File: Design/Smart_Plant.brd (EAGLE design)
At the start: 80 x 129.1 mm, 69 parts, among them IC1 TP4056, IC2 TLC555CDR, IC3 AHT20, IC4 RT9080-33GJ5, J6 USB-C, Q1 IRLML0100, T1 MMBT2222A, T2 LBSS84LT1G, U2 ESP32-WROOM-32

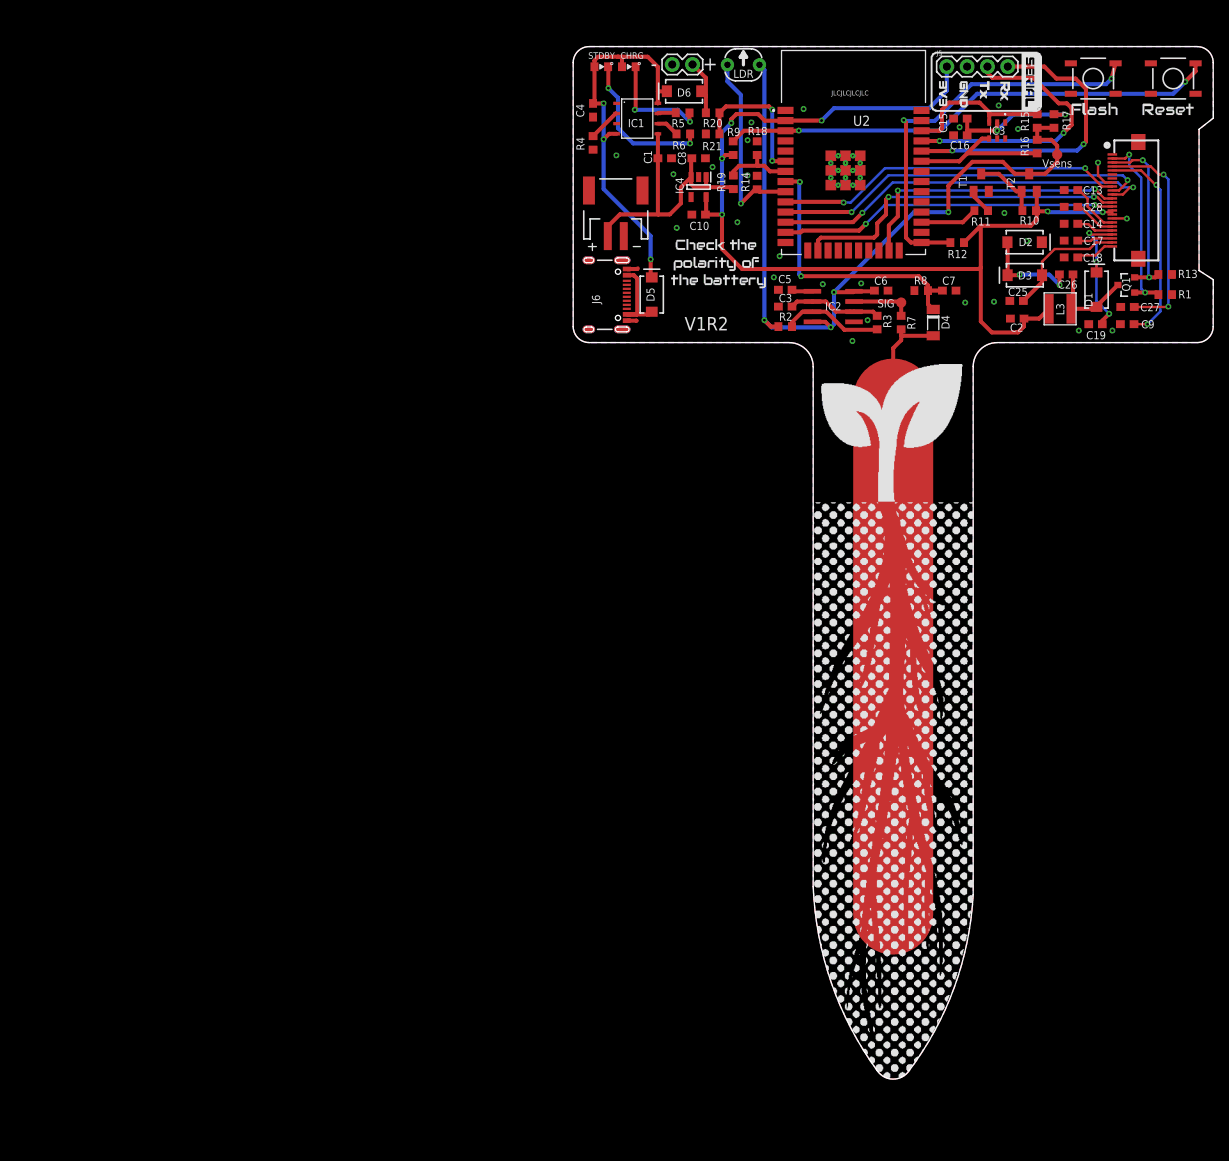
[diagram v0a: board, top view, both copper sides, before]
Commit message: SoC first draft
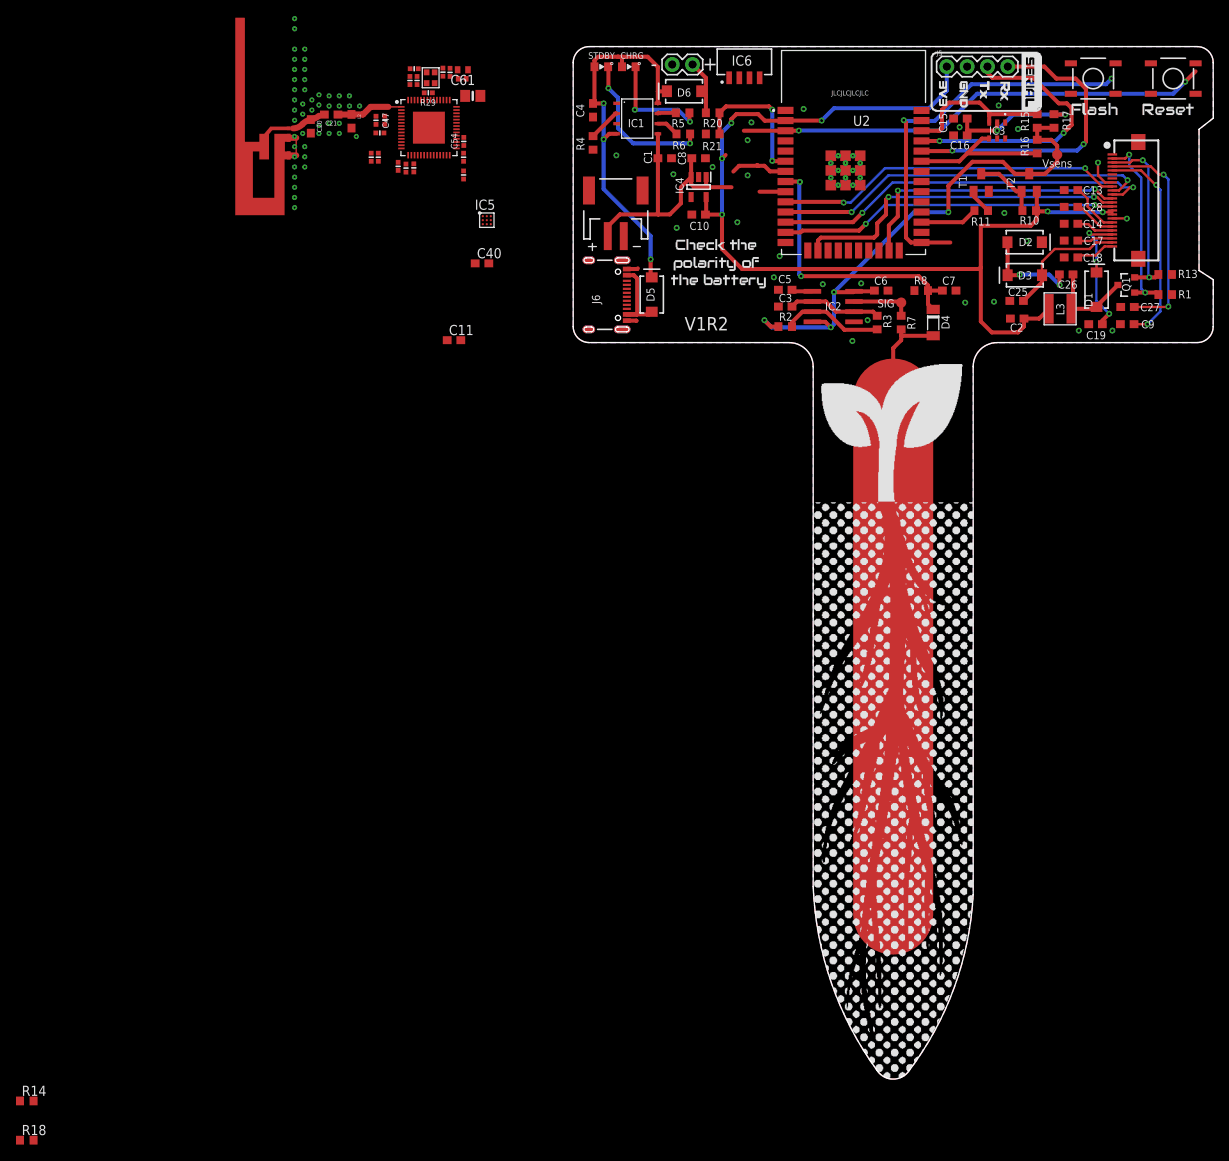
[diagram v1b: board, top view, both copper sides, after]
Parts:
- removed LDR: PHOTOCELLPTH, SparkFun-Sensors:PHOTOCELL
- removed R12: 10k, rcl:R0603
- removed R19: 1M, rcl:R0603
- removed R9: 10K, rcl:R0603
- added C11: 100nF, rcl:C0603
- added C20: 2.4pF, esp32-thing-temp:0603
- added C21: 5.6pF, esp32-thing-temp:0603
- added C40: 1uF, rcl:C0603
- added C46, C48, C55, C57, C62, C63: 1uF, microbuilder:_0402NO
- added C47, C52, C53, C54, C56, C58: 0.1uF, microbuilder:_0402NO
- added C49: 22uF, microbuilder:0805-NO
- added C59, C60: 16pF, microbuilder:_0402NO
- added C61: 1uF, SpaceDIY_passive_components:C0402
- added E2: ANTENNA, esp32-thing-temp:TRACE_ANTENNA_2.4GHZ_25.7MM_TUNED
- added IC5: LC709203F/MH, adafruit_sensor:WLCSP9
- added IC6: VEML7700-TR, SpaceDIY_sensors:VEML7700
- added L2: 2.7nH, SparkFun-Passives:0603
- added L5: 2nH, microbuilder:_0402NO
- added R29: 0, microbuilder:_0402NO
- added R30: 1Meg, microbuilder:_0402NO
- added R31: 10K, SpaceDIY_passive_components:R0402
- added U$42: (no value), itsy_silks:QTPY_ESP32_TOP
- added X5: ESP32-S3QFN54, adafruit_wireless:QFN56_7X7
- added Y2: 40MHz, microbuilder:CRYSTAL_2X1.6
- R14: value 10k -> 1M
- moved R18 154.0 mm to (-68.3, -99.7), turned to 0 degrees
- moved R14 146.7 mm to (-68.3, -94.8), turned to 0 degrees
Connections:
- new net !RESET: C61.1, R31.2, S2.3, X5.4
- new net A2: X5.14
- new net A3: X5.13
- new net IO10_DBLTAP: C62.1, R30.2, X5.15
- new net LNA_IN1: C21.1, L2.1, X5.1
- new net MISO: X5.42
- new net N$53: C59.1, X5.54, Y2.3
- new net N$54: C60.1, R29.1, Y2.1
- new net N$55: R29.2, X5.53
- new net NEOPIX: X5.44
- new net NEOPIX_PWR: X5.43
- new net SCK: X5.41
- new net SCL1: X5.45
- new net SDA1: X5.47
- new net TRACE_ANT1: C20.1, C21.2, E2.ANT
- new net VDD3P3: C47.1, L5.2, X5.2, X5.3
- new net VDD_SPI: C54.1, C55.1, X5.29
- net 3.3V: now also C46.1, C48.1, C49.1, C52.1, C53.1, C56.1, C57.1, C58.1, C63.1, L5.1, R31.1, X5.20, X5.27, X5.46, X5.55, X5.56; no longer R12.1, R9.2
- net BATTERY: now also R14.2, X5.24; no longer R19.2
- net D+: now also X5.26
- net D-: now also X5.25
- net GND: now also C11.2, C20.2, C40.2, C46.2, C47.2, C48.2, C49.2, C52.2, C53.2, C54.2, C55.2, C56.2, C57.2, C58.2, C59.2, C60.2, C61.2, C62.2, C63.2, E2.GND, E2.GND2, IC5.A1, IC5.B1, IC6.3, L2.2, R30.1, X5.57; no longer R14.2
- net IO0: now also X5.5; no longer R12.2
- net LIGHT: no longer LDR.1, R14.1
- net MOISTURE: now also X5.23
- net MOSI: now also X5.40
- net RST: no longer R9.1, S2.3
- net RX: now also X5.50
- net SCL: now also IC5.C2, IC6.1, X5.11
- net SDA: now also IC5.C1, IC6.4, X5.12
- net SENS: now also X5.9
- net TX: now also X5.49
- net VBAT: now also C40.1, IC5.A3, R14.1; no longer R19.1
- net VSENS: now also C11.1, IC6.2; no longer LDR.2
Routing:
- net VSENS: track 101.5 -> 69.3 mm
- net LIGHT: track 24.5 -> 3.25 mm, vias 1 -> 0
- net LNA_IN1: track 0.00 -> 8.01 mm
- net GND: track 8.21 -> 12.3 mm, vias 26 -> 73
- net 3.3V: track 135.0 -> 131.1 mm
- net TRACE_ANT1: track 0.00 -> 3.59 mm
- net RST: track 62.4 -> 59.5 mm
- net IO0: track 50.9 -> 48.9 mm
- net BATTERY: track 8.99 -> 7.25 mm
- added copper zone on layer 15, net 3.3V
- added copper zone on layer 2, net GND

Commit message: Design V1R3
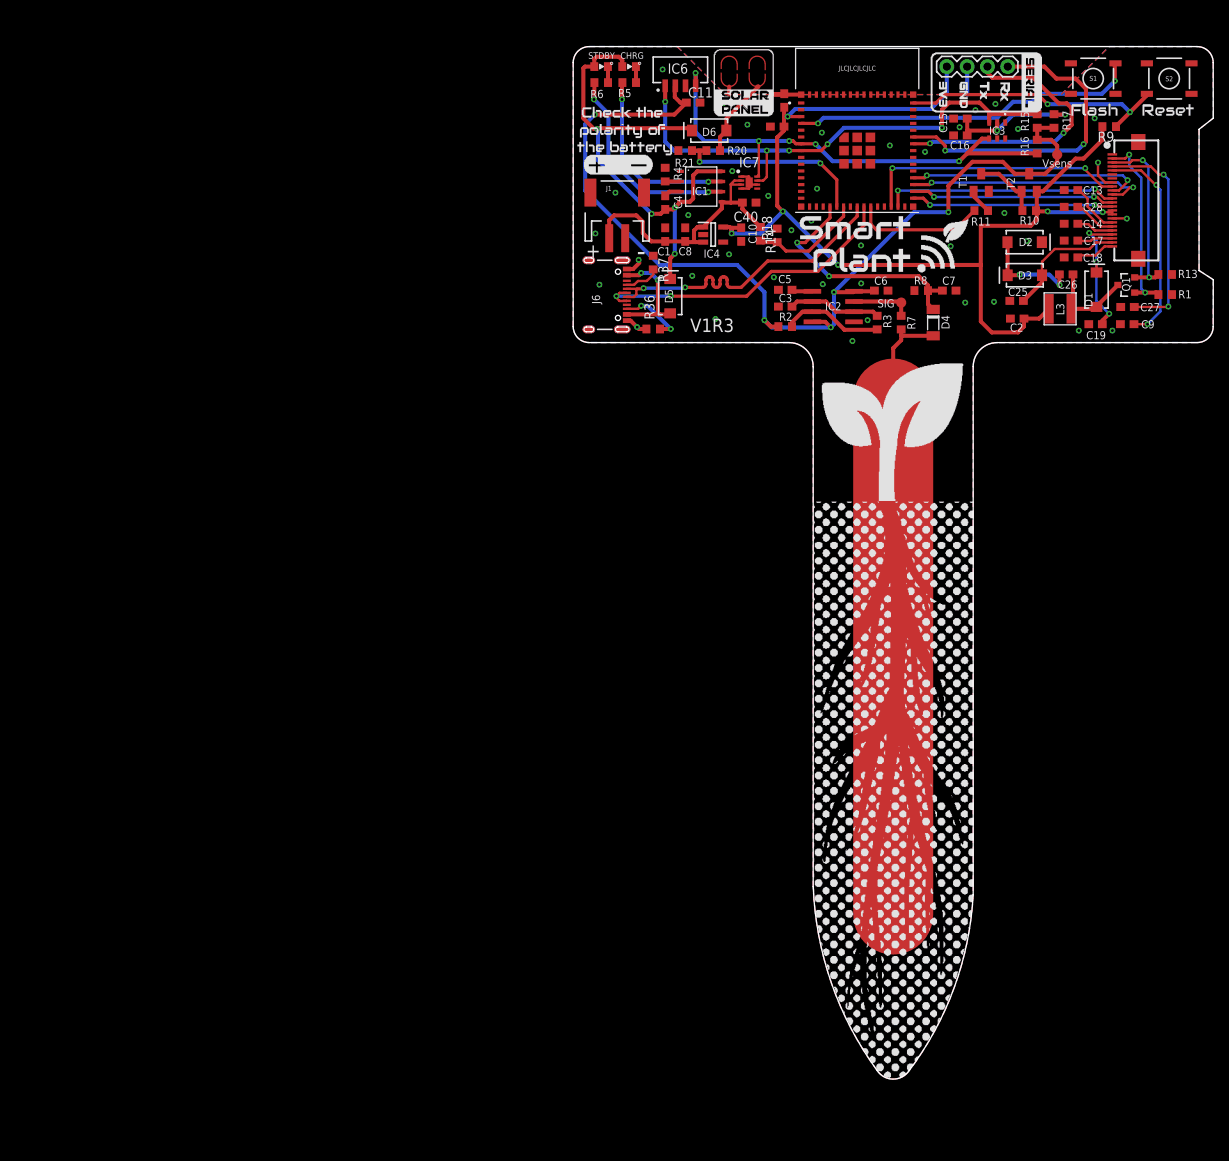
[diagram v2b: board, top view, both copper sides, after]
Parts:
- removed C21: 5.6pF, esp32-thing-temp:0603
- removed C46, C48, C55, C57, C62, C63: 1uF, microbuilder:_0402NO
- removed C47, C52, C53, C54, C56, C58: 0.1uF, microbuilder:_0402NO
- removed C49: 22uF, microbuilder:0805-NO
- removed C59, C60: 16pF, microbuilder:_0402NO
- removed C61: 1uF, SpaceDIY_passive_components:C0402
- removed E2: ANTENNA, esp32-thing-temp:TRACE_ANTENNA_2.4GHZ_25.7MM_TUNED
- removed IC5: LC709203F/MH, adafruit_sensor:WLCSP9
- removed J4: (no value), SpaceDIY_connectors:JST-2-SMD
- removed L2: 2.7nH, SparkFun-Passives:0603
- removed L5: 2nH, microbuilder:_0402NO
- removed R29: 0, microbuilder:_0402NO
- removed R30: 1Meg, microbuilder:_0402NO
- removed R31: 10K, SpaceDIY_passive_components:R0402
- removed U$42: (no value), itsy_silks:QTPY_ESP32_TOP
- removed U2: ESP32-WROOM-32, ESP32-WROOM-32:MODULE_ESP32-WROOM-32
- removed X5: ESP32-S3QFN54, adafruit_wireless:QFN56_7X7
- removed Y2: 40MHz, microbuilder:CRYSTAL_2X1.6
- added C12: 0.1uF, rcl:C0603
- added IC7: MAX17048G+T10, SpaceDIY_IC:SON50P200X200X80-9N
- added R36, R37: 5.1k, rcl:R0603
- added R9: 10K, rcl:R0603
- added U1: ESP32-S3-MINI-1-N8, SpaceDIY_modules:XCVR_ESP32-S3-MINI-1-N8
- C20: value 2.4pF -> 10uF; device esp32-thing-temp:0603 -> rcl:C0603
- C40: value 1uF -> 0.1uF
- FPC: device SpaceDIY_connectors:FPC-05FB-24PH20 -> SpaceDIY_connectors:FPC_24_0.5MM
- J1: device SparkFun-Connectors:1X02 -> SpaceDIY_connectors:JST-2-SMD
- moved R18 146.9 mm to (25.5, 13.4), turned to 90 degrees
- moved R14 142.0 mm to (23.4, 13.6), turned to 270 degrees
- moved C20 58.3 mm to (25.5, 27.0), turned to 180 degrees
- moved C11 42.1 mm to (15.0, 30.0)
- moved C40 34.3 mm to (22.0, 17.5)
- moved J1 20.1 mm to (5.50, 17.0)
- moved C4 14.6 mm to (11.5, 17.5), turned to 90 degrees
- moved R6 12.1 mm to (3.50, 32.5)
- moved IC1 11.7 mm to (16.0, 19.5)
- moved R4 9.85 mm to (11.5, 21.0), turned to 270 degrees
- moved C8 9.69 mm to (14.0, 13.5), turned to 90 degrees
- moved C1 9.54 mm to (11.5, 13.5), turned to 90 degrees
- moved IC6 8.06 mm to (10.0, 32.5)
- moved R5 7.68 mm to (7.00, 32.5)
- moved IC4 6.21 mm to (17.5, 13.5), turned to 0 degrees
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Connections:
- removed net !RESET: C61.1, R31.2, S2.3, X5.4
- removed net A2: X5.14
- removed net A3: X5.13
- removed net IO10_DBLTAP: C62.1, R30.2, X5.15
- removed net LIGHT: U2.9
- removed net LNA_IN1: C21.1, L2.1, X5.1
- removed net MISO: X5.42
- removed net N$53: C59.1, X5.54, Y2.3
- removed net N$54: C60.1, R29.1, Y2.1
- removed net N$55: R29.2, X5.53
- removed net NEOPIX: X5.44
- removed net NEOPIX_PWR: X5.43
- removed net SCK: X5.41
- removed net SCL1: X5.45
- removed net SDA1: X5.47
- removed net TRACE_ANT1: C20.1, C21.2, E2.ANT
- removed net VDD3P3: C47.1, L5.2, X5.2, X5.3
- removed net VDD_SPI: C54.1, C55.1, X5.29
- new net +SOL: D6.A, R20.1
- new net N$35: J6.B5, R36.2
- net 3.3V: now also C12.1, C20.1, R9.2, U1.3; no longer C46.1, C48.1, C49.1, C52.1, C53.1, C56.1, C57.1, C58.1, C63.1, L5.1, R31.1, U2.2, X5.20, X5.27, X5.46, X5.55, X5.56
- net BATTERY: now also U1.21; no longer U2.7, X5.24
- net BUSY: now also U1.28; no longer U2.10
- net D+: now also U1.24; no longer X5.26
- net D-: now also U1.23; no longer X5.25
- net DC: now also U1.33; no longer U2.12
- net DISPCS: now also U1.29; no longer U2.23
- net GND: now also C12.2, IC7.1, IC7.4, IC7.6, IC7.9, R36.1, R37.1, U1.1, U1.2, U1.42, U1.43, U1.46, U1.47, U1.48, U1.49, U1.50, U1.51, U1.52, U1.53, U1.54, U1.55, U1.56, U1.57, U1.58, U1.59, U1.60, U1.61, U1.61_1, U1.61_2, U1.61_3, U1.61_4, U1.61_5, U1.61_6, U1.61_7, U1.61_8, U1.62, U1.63, U1.64, U1.65; no longer C46.2, C47.2, C48.2, C49.2, C52.2, C53.2, C54.2, C55.2, C56.2, C57.2, C58.2, C59.2, C60.2, C61.2, C62.2, C63.2, E2.GND, E2.GND2, IC5.A1, IC5.B1, J4.2, L2.2, R30.1, U2.1, U2.15, U2.38, U2.39_1, U2.39_10, U2.39_11, U2.39_12, U2.39_13, U2.39_14, U2.39_15, U2.39_16, U2.39_17, U2.39_18, U2.39_19, U2.39_2, U2.39_20, U2.39_21, U2.39_3, U2.39_4, U2.39_5, U2.39_6, U2.39_7, U2.39_8, U2.39_9, X5.57
- net IO0: now also U1.4; no longer U2.25, X5.5
- net MOISTURE: now also U1.19; no longer U2.8, X5.23
- net MOSI: now also U1.31; no longer U2.13, X5.40
- net N$46: now also J6.A5, R37.2; no longer D6.A, J1.1, R20.1
- net RESET: now also U1.34; no longer U2.11
- net RST: now also R9.1, S2.3, U1.45; no longer U2.3
- net RX: now also U1.40; no longer U2.34, X5.50
- net SCL: now also IC7.7, U1.8; no longer IC5.C2, U2.36, X5.11
- net SCLK: now also U1.32; no longer U2.16
- net SDA: now also IC7.8, U1.7; no longer IC5.C1, U2.33, X5.12
- net SENS: now also U1.25; no longer U2.27, X5.9
- net TX: now also U1.39; no longer U2.35, X5.49
- net VBAT: now also IC7.2, IC7.3, J1.1; no longer IC5.A3, J4.1
- net VSOLAR: now also U1.20; no longer U2.6
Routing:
- net VSENS: track 69.3 -> 125.7 mm, vias 4 -> 5
- net SCL: track 19.1 -> 64.3 mm, vias 0 -> 5
- net SDA: track 18.4 -> 61.7 mm, vias 0 -> 5
- net D+: track 0.00 -> 40.1 mm, vias 0 -> 2
- net D-: track 0.00 -> 39.3 mm, vias 0 -> 2
- net RST: track 59.5 -> 34.1 mm
- net N$1: track 2.86 -> 26.2 mm, vias 0 -> 2
- net N$6: track 2.29 -> 23.3 mm, vias 0 -> 2
- net DC: track 48.7 -> 30.8 mm
- net RESET: track 47.5 -> 29.7 mm
- net N$3: track 19.2 -> 2.00 mm, vias 2 -> 0
- net SCLK: track 42.5 -> 25.5 mm
- net MOSI: track 42.3 -> 25.3 mm
- net GND: track 12.3 -> 26.9 mm, vias 73 -> 40
- net VIN: track 48.7 -> 62.8 mm, vias 3 -> 4
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- added copper zone on layer 1, net +SOL
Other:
- board text added: "V1R3"
- board text removed: "+"
- board text removed: "-"
- board text removed: "V1R2"
